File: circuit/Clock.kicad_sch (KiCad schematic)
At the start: 16 parts, among them J1 Conn_01x06_Pin, U1 WeMos_S2_mini, U2 ESP32-S3-ZERO

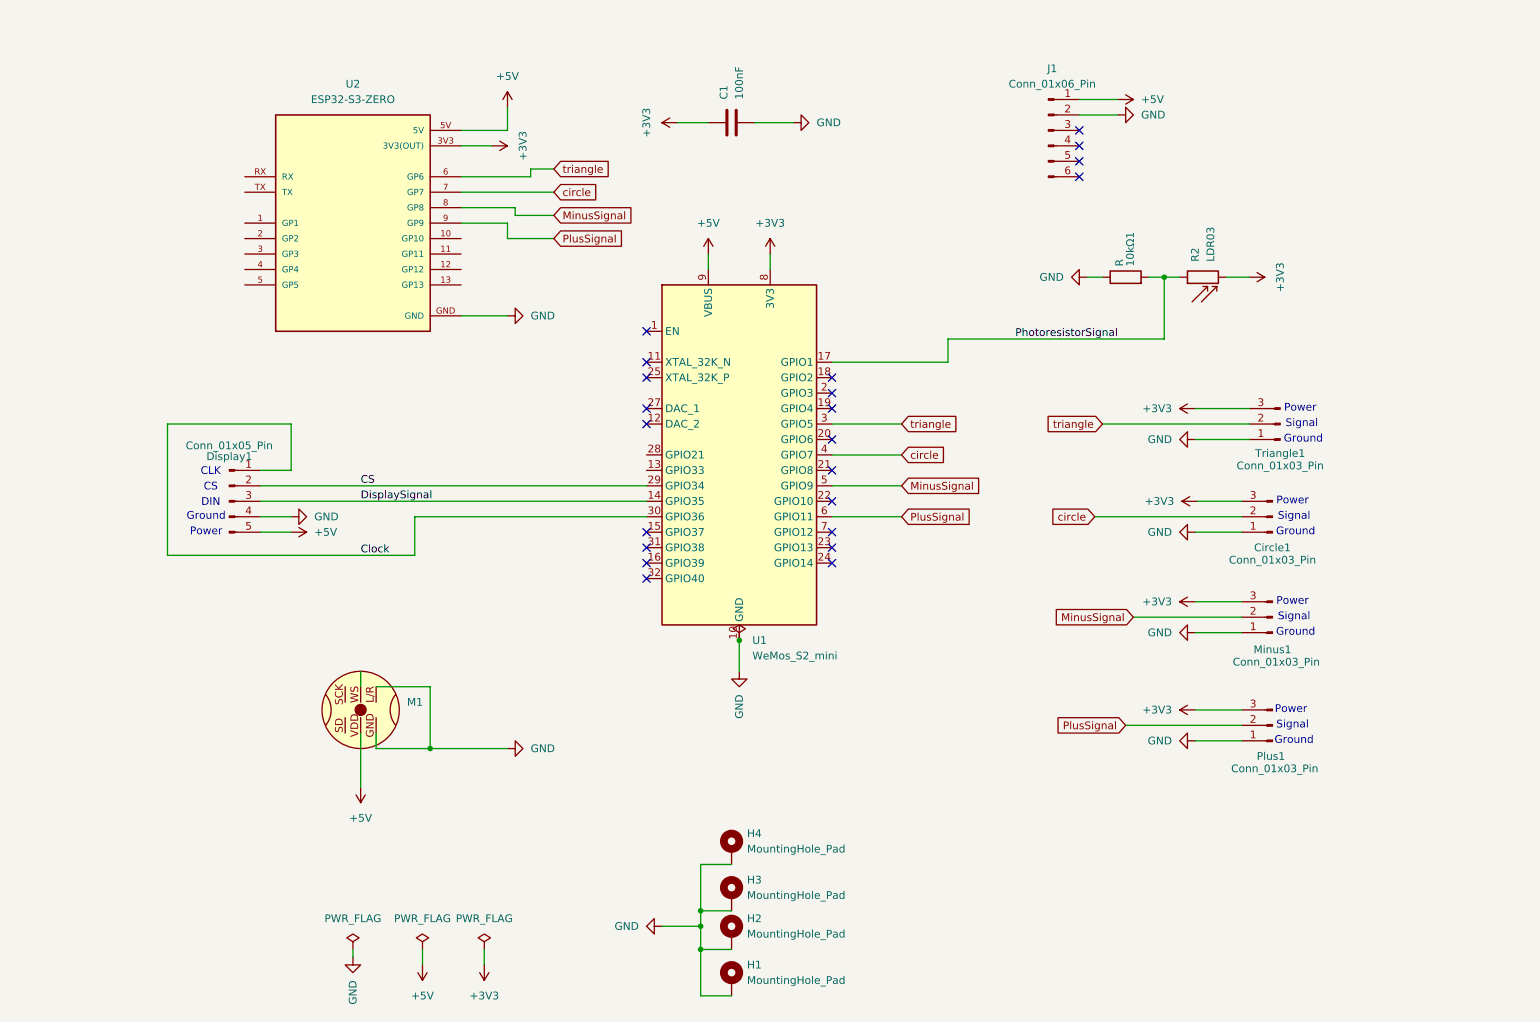
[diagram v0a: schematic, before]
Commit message: updated pcb
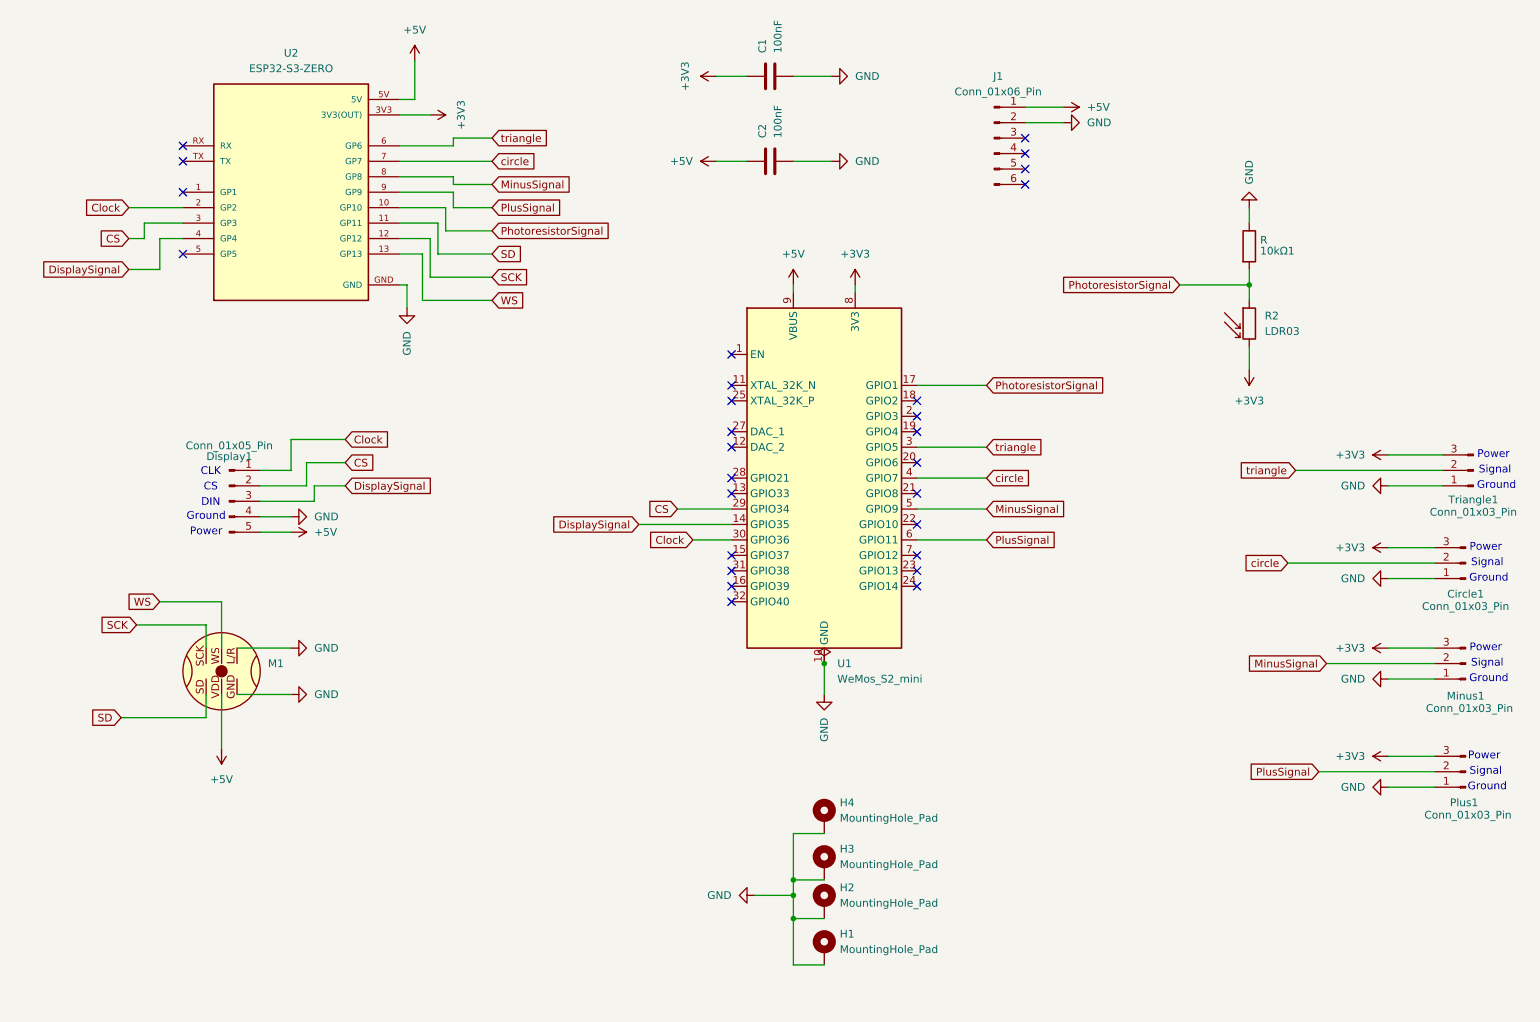
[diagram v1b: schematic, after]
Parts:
- added C2: 100nF, Capacitor_THT:C_Disc_D8.0mm_W2.5mm_P5.00mm, symbol Device:C
- U1: footprint Module:WEMOS_S2_mini -> wemos2:wemoss2
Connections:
- net +5V: now also C2.1
- net CS: now also U2.3 (GP3)
- net Clock: now also U2.2 (GP2)
- net DisplaySignal: now also U2.4 (GP4)
- net GND: now also C2.2
- net PhotoresistorSignal: now also U2.10 (GP10)
- net SD: now reaches U2.11 (GP11)
- net SD: now also M1.SD
- net SCK: now reaches U2.12 (GP12)
- net SCK: now also M1.SCK
- net WS: now reaches U2.13 (GP13)
- net WS: now also M1.WS
- no-connect marks 22 -> 28
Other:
- moved on the sheet: 10kΩ1, C1, Circle1, H1, H2, H3, H4, J1, M1, Minus1, Plus1, R2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
